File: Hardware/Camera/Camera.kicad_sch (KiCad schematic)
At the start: 66 parts, among them J1 Power, J2 ICC Out, J3 USB_B_Mini, J4 SWDIO, J5 Header Pins, J6 Camer Interface, Q1 AO3401A, SW1 SW_SPDT, U1 STM32F407ZGT6, U2 LM317L_SOT-89, U3 LM317L_SOT-89, Y1 16MHz

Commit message: Optimizing camera placement
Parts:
- J6: footprint Connector_PinHeader_1.00mm:PinHeader_1x24_P1.00mm_Vertical_SMD_Pin1Left -> Lib:SAMTEC_ZF5S-24-01-T-WT
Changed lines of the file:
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@@
       (effects (font (size 1.27 1.27)) (justify left))
     )
-    (property "Footprint" "Connector_PinHeader_1.00mm:PinHeader_1x24_P1.00mm_Vertical_SMD_Pin1Left" (id 2) (at 295.91 130.81 0)
+    (property "Footprint" "Lib:SAMTEC_ZF5S-24-01-T-WT" (id 2) (at 295.91 130.81 0)
       (effects (font (size 1.27 1.27)) hide)
     )
@@
     )
     (path "/701033a6-4188-46b9-b56d-63cc408b62d6"
-      (reference "J6") (unit 1) (value "Camer Interface") (footprint "Connector_PinHeader_1.00mm:PinHeader_1x24_P1.00mm_Vertical_SMD_Pin1Left")
+      (reference "J6") (unit 1) (value "Camer Interface") (footprint "Lib:SAMTEC_ZF5S-24-01-T-WT")
     )
     (path "/788a04c2-6e94-4f16-bd0e-64642763e556"

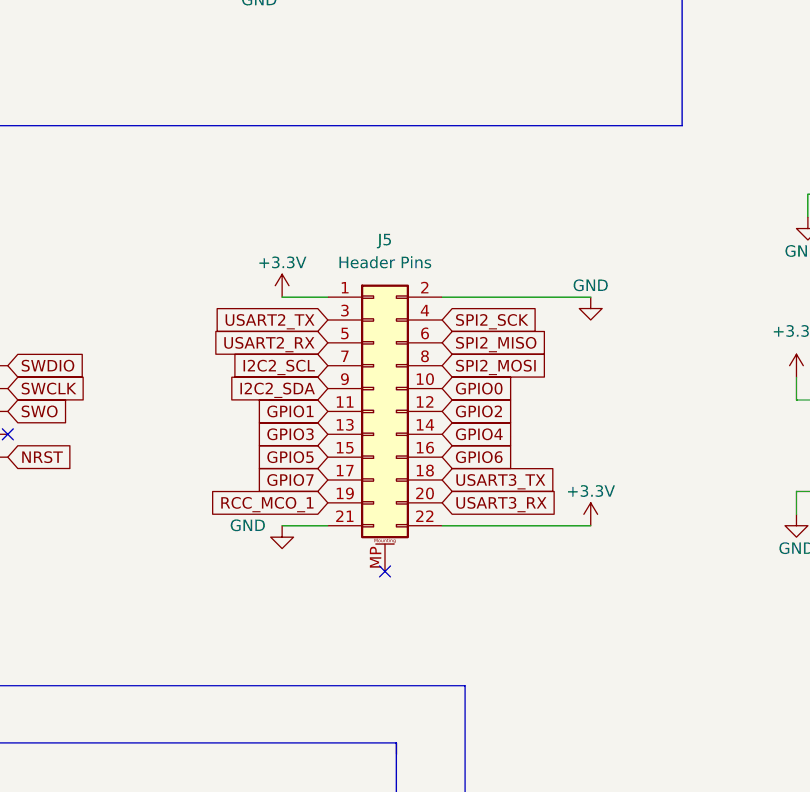
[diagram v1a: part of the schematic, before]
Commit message: Basic routing done
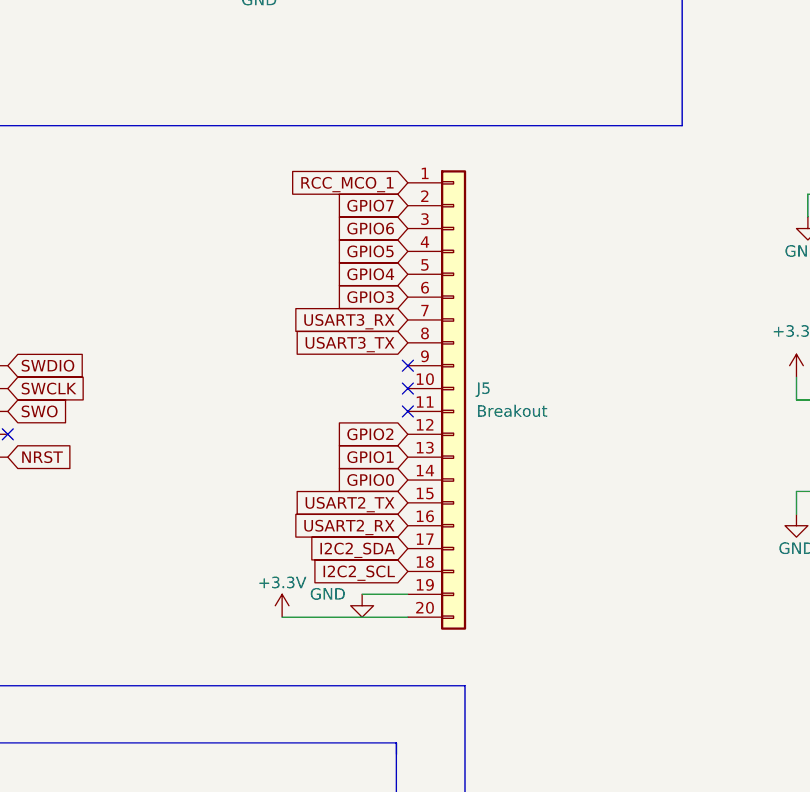
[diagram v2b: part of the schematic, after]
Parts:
- removed J5: Header Pins, Connector_PinHeader_1.27mm:PinHeader_2x11_P1.27mm_Vertical_SMD, symbol Connector_Generic_MountingPin:Conn_02x11_Odd_Even_MountingPin
- added J5: Breakout, Connector_PinHeader_1.27mm:PinHeader_1x20_P1.27mm_Vertical, symbol Connector_Generic:Conn_01x20
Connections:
- net +3V3: now also J5.20 (Pin_20)
- net GND: now also J5.19 (Pin_19)
- net GPIO0: now also J5.14 (Pin_14)
- net GPIO1: now also J5.13 (Pin_13)
- net GPIO2: now also J5.12 (Pin_12)
- net GPIO3: now also J5.6 (Pin_6)
- net GPIO4: now also J5.5 (Pin_5)
- net GPIO5: now also J5.4 (Pin_4)
- net GPIO6: now also J5.3 (Pin_3)
- net GPIO7: now also J5.2 (Pin_2)
- net I2C2_SCL: now also J5.18 (Pin_18)
- net I2C2_SDA: now also J5.17 (Pin_17)
- net RCC_MCO_1: now also J5.1 (Pin_1)
- net USART2_RX: now also J5.16 (Pin_16)
- net USART2_TX: now also J5.15 (Pin_15)
- net USART3_RX: now also J5.7 (Pin_7)
- net USART3_TX: now also J5.8 (Pin_8)
- no-connect marks 73 -> 75

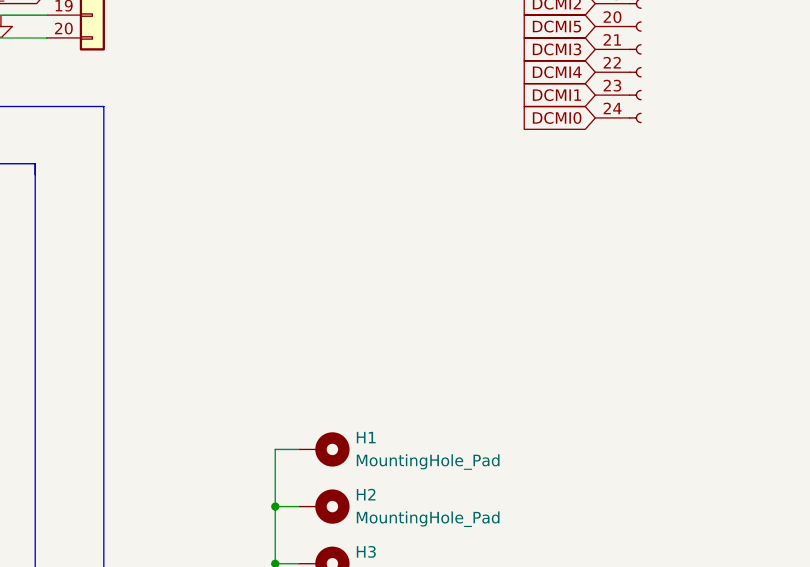
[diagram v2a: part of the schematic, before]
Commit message: About to re-do layout
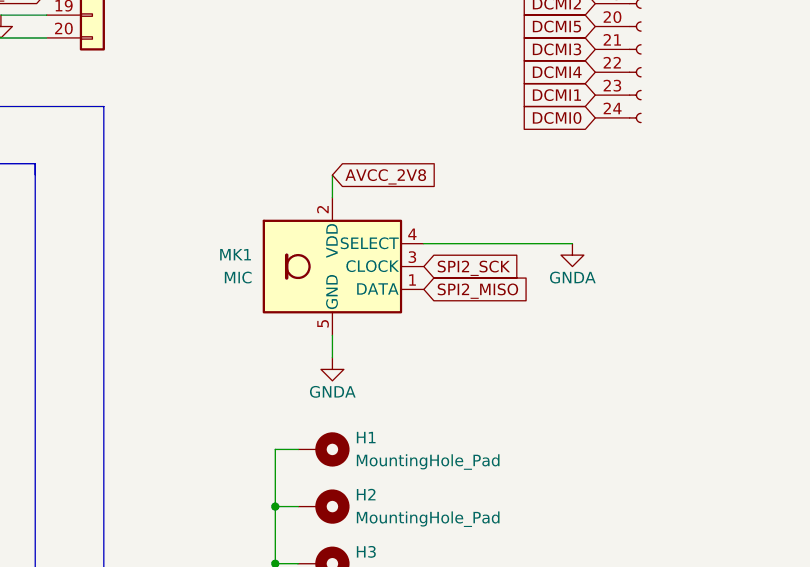
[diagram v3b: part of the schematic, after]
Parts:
- added MK1: MIC, Sensor_Audio:Infineon_PG-LLGA-5-1, symbol Sensor_Audio:IM69D130
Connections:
- net AVCC_2V8: now also MK1.2 (VDD)
- net GND: now also MK1.4 (SELECT), MK1.5 (GND)
- net SPI2_MISO: now also MK1.1 (DATA)
- net SPI2_SCK: now also MK1.3 (CLOCK)
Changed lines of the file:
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@@
   (no_connect (at 43.18 377.19))
   (no_connect (at 93.98 139.7))
+  (wire (pts (xy 261.62 187.96) (xy 261.62 185.42))
+    (stroke (width 0) (type default) (color 0 0 0 0))
+  )
   (wire (pts (xy 138.43 58.42) (xy 148.59 58.42))
     (stroke (width 0) (type default) (color 0 0 0 0))
@@
     (stroke (width 0) (type default) (color 0 0 0 0))
   )
+  (wire (pts (xy 261.62 167.64) (xy 261.62 170.18))
+    (stroke (width 0) (type default) (color 0 0 0 0))
+  )
   (wire (pts (xy 60.96 204.47) (xy 60.96 207.01))
     (stroke (width 0) (type default) (color 0 0 0 0))
@@
     (stroke (width 0) (type default) (color 0 0 0 0))
   )
+  (wire (pts (xy 271.78 175.26) (xy 288.29 175.26))
+    (stroke (width 0) (type default) (color 0 0 0 0))
+  )
   (wire (pts (xy 151.13 33.02) (xy 151.13 35.56))
     (stroke (width 0) (type default) (color 0 0 0 0))
@@
     )
   )
+  (global_label "AVCC_2V8" (shape input) (at 261.62 167.64 0) (fields_autoplaced)
+    (effects (font (size 1.27 1.27)) (justify left))
+    (property "Intersheet References" "${INTERSHEET_REFS}" (id 0) (at 273.2255 167.5606 0)
+      (effects (font (size 1.27 1.27)) (justify left) hide)
+    )
+  )
   (global_label "USART3_TX" (shape input) (at 229.87 121.92 180) (fields_autoplaced)
     (effects (font (size 1.27 1.27)) (justify right))
@@
     )
   )
+  (global_label "SPI2_MISO" (shape input) (at 271.78 180.34 0) (fields_autoplaced)
+    (effects (font (size 1.27 1.27)) (justify left))
+    (property "Intersheet References" "${INTERSHEET_REFS}" (id 0) (at 284.0507 180.2606 0)
+      (effects (font (size 1.27 1.27)) (justify left) hide)
+    )
+  )
   (global_label "DCMI_VSYNC" (shape input) (at 290.83 118.11 180) (fields_autoplaced)
     (effects (font (size 1.27 1.27)) (justify right))
@@
     )
   )
+  (global_label "SPI2_SCK" (shape input) (at 271.78 177.8 0) (fields_autoplaced)
+    (effects (font (size 1.27 1.27)) (justify left))
+    (property "Intersheet References" "${INTERSHEET_REFS}" (id 0) (at 283.2041 177.7206 0)
+      (effects (font (size 1.27 1.27)) (justify left) hide)
+    )
+  )
   (global_label "I2C2_SDA" (shape input) (at 43.18 300.99 180) (fields_autoplaced)
     (effects (font (size 1.27 1.27)) (justify right))
@@
     (pin "1")
   )
+  (symbol (lib_id "Sensor_Audio:IM69D130") (at 261.62 177.8 0) (unit 1)
+    (in_bom yes) (on_board yes) (fields_autoplaced)
+    (property "Reference" "MK1" (id 0) (at 252.73 176.5299 0)
+      (effects (font (size 1.27 1.27)) (justify right))
+    )
+    (property "Value" "MIC" (id 1) (at 252.73 179.0699 0)
+      (effects (font (size 1.27 1.27)) (justify right))
+    )
+    (property "Footprint" "Sensor_Audio:Infineon_PG-LLGA-5-1" (id 2) (at 279.4 185.42 0)
+      (effects (font (size 1.27 1.27) italic) hide)
+    )
+    (property "Datasheet" "https://www.infineon.com/dgdl/Infineon-IM69D130-DS-v01_00-EN.pdf?fileId=5546d462602a9dc801607a0e46511a2e" (id 3) (at 261.62 177.8 0)
+      (effects (font (size 1.27 1.27)) hide)
+    )
+    (pin "1")
+    (pin "2")
+    (pin "3")
+    (pin "4")
+    (pin "5")
+  )
   (symbol (lib_id "Device:C_Small") (at 139.7 189.23 0) (unit 1)
     (in_bom yes) (on_board yes) (fields_autoplaced)
@@
     (pin "2")
   )
+  (symbol (lib_id "power:GNDA") (at 261.62 187.96 0) (unit 1)
+    (in_bom yes) (on_board yes)
+    (property "Reference" "#PWR054" (id 0) (at 261.62 194.31 0)
+      (effects (font (size 1.27 1.27)) hide)
+    )
+    (property "Value" "GNDA" (id 1) (at 261.62 191.77 0))
+    (property "Footprint" "" (id 2) (at 261.62 187.96 0)
+      (effects (font (size 1.27 1.27)) hide)
+    )
+    (property "Datasheet" "" (id 3) (at 261.62 187.96 0)
+      (effects (font (size 1.27 1.27)) hide)
+    )
+    (pin "1")
+  )
   (symbol (lib_id "Device:D_Schottky") (at 58.42 22.86 90) (unit 1)
     (in_bom yes) (on_board yes) (fields_autoplaced)
@@
     (pin "1")
   )
+  (symbol (lib_id "power:GNDA") (at 288.29 175.26 0) (unit 1)
+    (in_bom yes) (on_board yes)
+    (property "Reference" "#PWR055" (id 0) (at 288.29 181.61 0)
+      (effects (font (size 1.27 1.27)) hide)
+    )
+    (property "Value" "GNDA" (id 1) (at 288.29 179.07 0))
+    (property "Footprint" "" (id 2) (at 288.29 175.26 0)
+      (effects (font (size 1.27 1.27)) hide)
+    )
+    (property "Datasheet" "" (id 3) (at 288.29 175.26 0)
+      (effects (font (size 1.27 1.27)) hide)
+    )
+    (pin "1")
+  )
   (symbol (lib_id "power:GND") (at 24.13 238.76 0) (unit 1)
     (in_bom yes) (on_board yes) (fields_autoplaced)
@@
       (reference "#PWR053") (unit 1) (value "GND") (footprint "")
     )
+    (path "/2cbb60b3-780c-4df0-85f4-a3eb01190307"
+      (reference "#PWR054") (unit 1) (value "GNDA") (footprint "")
+    )
+    (path "/965f769a-a693-48ab-b5f2-7607ed82b7ee"
+      (reference "#PWR055") (unit 1) (value "GNDA") (footprint "")
+    )
     (path "/92f31037-40e8-4176-8082-8041f0da9201"
       (reference "#PWR056") (unit 1) (value "GND") (footprint "")
@@
       (reference "L2") (unit 1) (value "39n") (footprint "Inductor_SMD:L_0603_1608Metric")
     )
+    (path "/12c7caee-e148-470b-9da2-ccaee29beb5f"
+      (reference "MK1") (unit 1) (value "MIC") (footprint "Sensor_Audio:Infineon_PG-LLGA-5-1")
+    )
     (path "/aa7af968-5118-421d-bd21-75f0ddb649f1"
